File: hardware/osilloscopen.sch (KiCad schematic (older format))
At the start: 59 parts, among them J1 SWD, J10 Conn_01x01_Male, J11 Conn_01x02_Male, J12 Conn_01x03_Male, J13 Conn_01x02_Male, J14 Conn_01x02_Male, J15 Conn_01x01_Male, J16 Conn_01x03_Male, J17 OLED, J18 GND, J19 VBAT, J2 OLED, J3 tip, J4 power, J5 Conn_01x03_Male, J6 Conn_01x01_Male, J7 Conn_01x04_Male, J8 Conn_01x01_Male, J9 Conn_01x03_Male, SW1 SW_Push, SW2 SW_Push, SW3 SW_Push, SW4 SW_Push, SW5 POWER, SW6 RESET, U1 AD623AN, U2 ICL7660, U3 STM32F103C8Tx, U4 AP1117-33, U5 XXX, Y1 Crystal

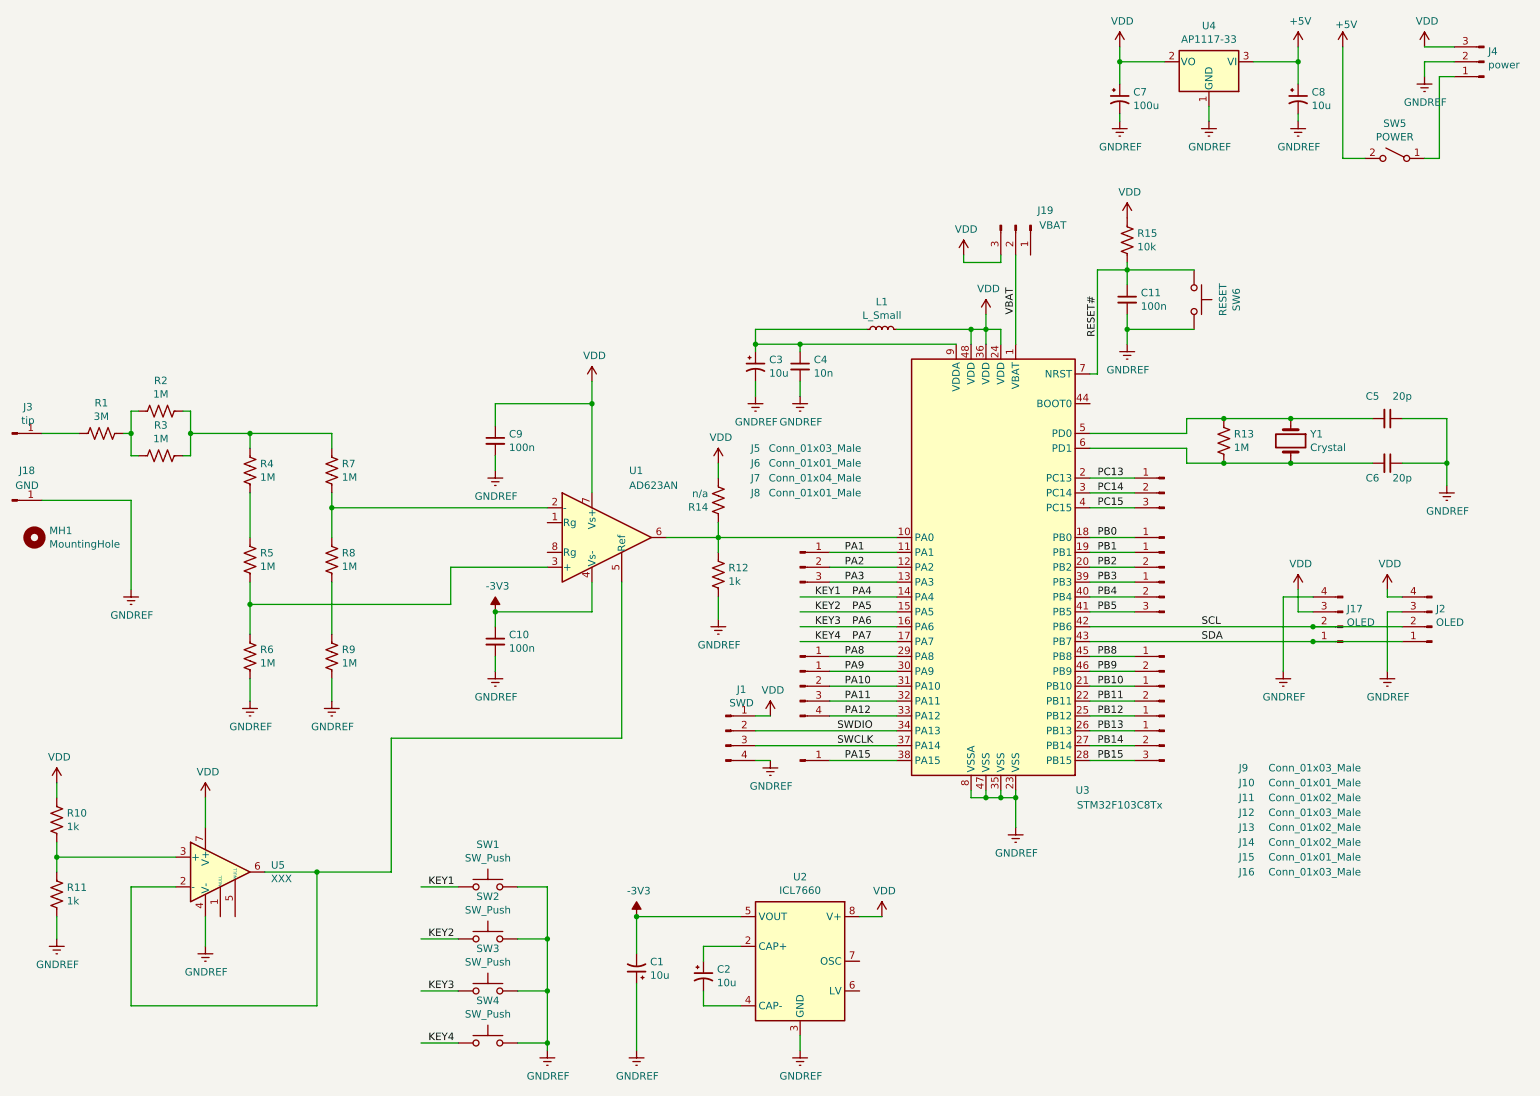
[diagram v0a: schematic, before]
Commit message: Add files via upload
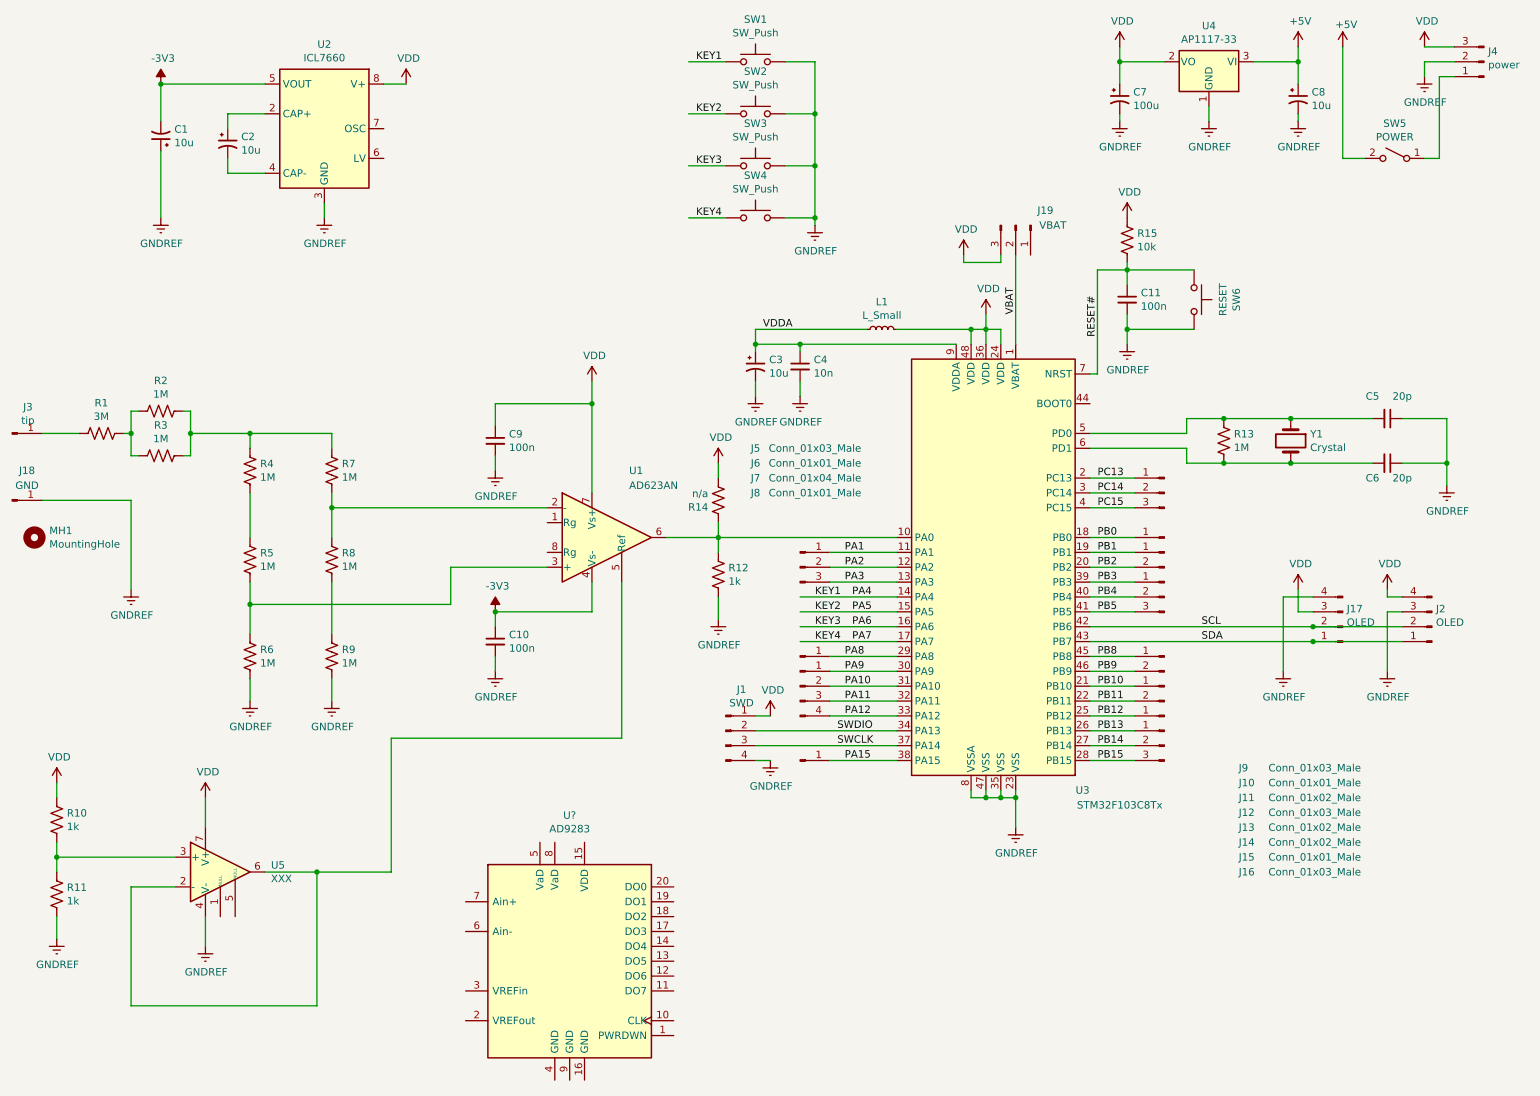
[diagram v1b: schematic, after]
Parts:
- added U?: AD9283, symbol Analog_ADC:AD9283
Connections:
- net labels added: VDDA
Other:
- moved on the sheet: C1, C2, SW1, SW2, SW3, SW4, U2
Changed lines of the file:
@@
 EESchema Schematic File Version 4
-LIBS:osilloscopen-cache
-EELAYER 26 0
+EELAYER 30 0
 EELAYER END
 $Descr A4 11693 8268
@@
 L Regulator_SwitchedCapacitor:ICL7660 U2
 U 1 1 5BCEDF67
-P 6300 6950
-F 0 "U2" H 6300 7517 50  0000 C CNN
-F 1 "ICL7660" H 6300 7426 50  0000 C CNN
-F 2 "Package_DIP:DIP-8_W7.62mm_LongPads" H 6400 6850 50  0001 C CNN
-F 3 "http://datasheets.maximintegrated.com/en/ds/ICL7660-MAX1044.pdf" H 6400 6850 50  0001 C CNN
-	1    6300 6950
+P 3100 1350
+F 0 "U2" H 3100 1917 50  0000 C CNN
+F 1 "ICL7660" H 3100 1826 50  0000 C CNN
+F 2 "Package_DIP:DIP-8_W7.62mm_LongPads" H 3200 1250 50  0001 C CNN
+F 3 "http://datasheets.maximintegrated.com/en/ds/ICL7660-MAX1044.pdf" H 3200 1250 50  0001 C CNN
+	1    3100 1350
 	-1   0    0    -1
 $EndComp
 Wire Wire Line
-	6700 6650 6850 6650
+	3500 1050 3650 1050
 $Comp
 L power:GNDREF #PWR0103
@@
 L power:GNDREF #PWR0105
 U 1 1 5BCEEDE7
-P 6300 7550
-F 0 "#PWR0105" H 6300 7300 50  0001 C CNN
-F 1 "GNDREF" H 6305 7377 50  0000 C CNN
-F 2 "" H 6300 7550 50  0001 C CNN
-F 3 "" H 6300 7550 50  0001 C CNN
-	1    6300 7550
-	1    0    0    -1
-$EndComp
-Wire Wire Line
-	6300 7550 6300 7450
+P 3100 1950
+F 0 "#PWR0105" H 3100 1700 50  0001 C CNN
+F 1 "GNDREF" H 3105 1777 50  0000 C CNN
+F 2 "" H 3100 1950 50  0001 C CNN
+F 3 "" H 3100 1950 50  0001 C CNN
+	1    3100 1950
+	1    0    0    -1
+$EndComp
+Wire Wire Line
+	3100 1950 3100 1850
 $Comp
 L Device:CP1_Small C2
 U 1 1 5BCEF09D
-P 5650 7050
-F 0 "C2" H 5741 7096 50  0000 L CNN
-F 1 "10u" H 5741 7005 50  0000 L CNN
-F 2 "Capacitor_THT:CP_Radial_D6.3mm_P2.50mm" H 5650 7050 50  0001 C CNN
-F 3 "~" H 5650 7050 50  0001 C CNN
-	1    5650 7050
+P 2450 1450
+F 0 "C2" H 2541 1496 50  0000 L CNN
+F 1 "10u" H 2541 1405 50  0000 L CNN
+F 2 "Capacitor_THT:CP_Radial_D6.3mm_P2.50mm" H 2450 1450 50  0001 C CNN
+F 3 "~" H 2450 1450 50  0001 C CNN
+	1    2450 1450
 	1    0    0    -1
 $EndComp
@@
 L Device:CP1_Small C1
 U 1 1 5BCEF0E8
-P 5200 7000
-F 0 "C1" H 5109 6954 50  0000 R CNN
-F 1 "10u" H 5109 7045 50  0000 R CNN
-F 2 "Capacitor_THT:CP_Radial_D6.3mm_P2.50mm" H 5200 7000 50  0001 C CNN
-F 3 "~" H 5200 7000 50  0001 C CNN
-	1    5200 7000
+P 2000 1400
+F 0 "C1" H 1909 1354 50  0000 R CNN
+F 1 "10u" H 1909 1445 50  0000 R CNN
+F 2 "Capacitor_THT:CP_Radial_D6.3mm_P2.50mm" H 2000 1400 50  0001 C CNN
+F 3 "~" H 2000 1400 50  0001 C CNN
+	1    2000 1400
 	-1   0    0    1
 $EndComp
 Wire Wire Line
-	5900 6850 5650 6850
-Wire Wire Line
-	5650 6850 5650 6950
-Wire Wire Line
-	5900 7250 5650 7250
-Wire Wire Line
-	5650 7250 5650 7150
+	2700 1250 2450 1250
+Wire Wire Line
+	2450 1250 2450 1350
+Wire Wire Line
+	2700 1650 2450 1650
+Wire Wire Line
+	2450 1650 2450 1550
 $Comp
 L power:GNDREF #PWR0106
 U 1 1 5BCEFBEB
-P 5200 7550
-F 0 "#PWR0106" H 5200 7300 50  0001 C CNN
-F 1 "GNDREF" H 5205 7377 50  0000 C CNN
-F 2 "" H 5200 7550 50  0001 C CNN
-F 3 "" H 5200 7550 50  0001 C CNN
-	1    5200 7550
+P 2000 1950
+F 0 "#PWR0106" H 2000 1700 50  0001 C CNN
+F 1 "GNDREF" H 2005 1777 50  0000 C CNN
+F 2 "" H 2000 1950 50  0001 C CNN
+F 3 "" H 2000 1950 50  0001 C CNN
+	1    2000 1950
 	1    0    0    -1
 $EndComp
@@
 L power:VDD #PWR0109
 U 1 1 5BCF1ECC
-P 6850 6650
-F 0 "#PWR0109" H 6850 6500 50  0001 C CNN
-F 1 "VDD" H 6867 6823 50  0000 C CNN
-F 2 "" H 6850 6650 50  0001 C CNN
-F 3 "" H 6850 6650 50  0001 C CNN
-	1    6850 6650
+P 3650 1050
+F 0 "#PWR0109" H 3650 900 50  0001 C CNN
+F 1 "VDD" H 3667 1223 50  0000 C CNN
+F 2 "" H 3650 1050 50  0001 C CNN
+F 3 "" H 3650 1050 50  0001 C CNN
+	1    3650 1050
 	1    0    0    -1
 $EndComp
@@
 L Switch:SW_Push SW1
 U 1 1 5BD06E7F
-P 4200 6450
-F 0 "SW1" H 4200 6735 50  0000 C CNN
-F 1 "SW_Push" H 4200 6644 50  0000 C CNN
-F 2 "Button_Switch_THT:SW_PUSH_6mm_H5mm" H 4200 6650 50  0001 C CNN
-F 3 "" H 4200 6650 50  0001 C CNN
-	1    4200 6450
+P 6000 900
+F 0 "SW1" H 6000 1185 50  0000 C CNN
+F 1 "SW_Push" H 6000 1094 50  0000 C CNN
+F 2 "Button_Switch_THT:SW_PUSH_6mm_H5mm" H 6000 1100 50  0001 C CNN
+F 3 "" H 6000 1100 50  0001 C CNN
+	1    6000 900
 	1    0    0    -1
 $EndComp
@@
 L Switch:SW_Push SW2
 U 1 1 5BD06EF3
-P 4200 6800
-F 0 "SW2" H 4200 7085 50  0000 C CNN
-F 1 "SW_Push" H 4200 6994 50  0000 C CNN
-F 2 "Button_Switch_THT:SW_PUSH_6mm_H5mm" H 4200 7000 50  0001 C CNN
-F 3 "" H 4200 7000 50  0001 C CNN
-	1    4200 6800
+P 6000 1250
+F 0 "SW2" H 6000 1535 50  0000 C CNN
+F 1 "SW_Push" H 6000 1444 50  0000 C CNN
+F 2 "Button_Switch_THT:SW_PUSH_6mm_H5mm" H 6000 1450 50  0001 C CNN
+F 3 "" H 6000 1450 50  0001 C CNN
+	1    6000 1250
 	1    0    0    -1
 $EndComp
@@
 L Switch:SW_Push SW3
 U 1 1 5BD06F40
-P 4200 7150
-F 0 "SW3" H 4200 7435 50  0000 C CNN
-F 1 "SW_Push" H 4200 7344 50  0000 C CNN
-F 2 "Button_Switch_THT:SW_PUSH_6mm_H5mm" H 4200 7350 50  0001 C CNN
-F 3 "" H 4200 7350 50  0001 C CNN
-	1    4200 7150
+P 6000 1600
+F 0 "SW3" H 6000 1885 50  0000 C CNN
+F 1 "SW_Push" H 6000 1794 50  0000 C CNN
+F 2 "Button_Switch_THT:SW_PUSH_6mm_H5mm" H 6000 1800 50  0001 C CNN
+F 3 "" H 6000 1800 50  0001 C CNN
+	1    6000 1600
 	1    0    0    -1
 $EndComp
@@
 L Switch:SW_Push SW4
 U 1 1 5BD06F8D
-P 4200 7500
-F 0 "SW4" H 4200 7785 50  0000 C CNN
-F 1 "SW_Push" H 4200 7694 50  0000 C CNN
-F 2 "Button_Switch_THT:SW_PUSH_6mm_H5mm" H 4200 7700 50  0001 C CNN
-F 3 "" H 4200 7700 50  0001 C CNN
-	1    4200 7500
-	1    0    0    -1
-$EndComp
-Wire Wire Line
-	4400 6450 4600 6450
-Wire Wire Line
-	4600 6450 4600 6800
-Wire Wire Line
-	4400 7500 4600 7500
-Connection ~ 4600 7500
-Wire Wire Line
-	4600 7500 4600 7550
-Wire Wire Line
-	4400 7150 4600 7150
-Connection ~ 4600 7150
-Wire Wire Line
-	4600 7150 4600 7500
-Wire Wire Line
-	4400 6800 4600 6800
-Connection ~ 4600 6800
-Wire Wire Line
-	4600 6800 4600 7150
+P 6000 1950
+F 0 "SW4" H 6000 2235 50  0000 C CNN
+F 1 "SW_Push" H 6000 2144 50  0000 C CNN
+F 2 "Button_Switch_THT:SW_PUSH_6mm_H5mm" H 6000 2150 50  0001 C CNN
+F 3 "" H 6000 2150 50  0001 C CNN
+	1    6000 1950
+	1    0    0    -1
+$EndComp
+Wire Wire Line
+	6200 900  6400 900
+Wire Wire Line
+	6400 900  6400 1250
+Wire Wire Line
+	6200 1950 6400 1950
+Connection ~ 6400 1950
+Wire Wire Line
+	6400 1950 6400 2000
+Wire Wire Line
+	6200 1600 6400 1600
+Connection ~ 6400 1600
+Wire Wire Line
+	6400 1600 6400 1950
+Wire Wire Line
+	6200 1250 6400 1250
+Connection ~ 6400 1250
+Wire Wire Line
+	6400 1250 6400 1600
 $Comp
 L power:GNDREF #PWR08
 U 1 1 5BD113E8
-P 4600 7550
-F 0 "#PWR08" H 4600 7300 50  0001 C CNN
-F 1 "GNDREF" H 4605 7377 50  0000 C CNN
-F 2 "" H 4600 7550 50  0001 C CNN
-F 3 "" H 4600 7550 50  0001 C CNN
-	1    4600 7550
-	1    0    0    -1
-$EndComp
-Wire Wire Line
-	4000 6450 3750 6450
-Wire Wire Line
-	4000 6800 3750 6800
-Wire Wire Line
-	4000 7150 3750 7150
-Wire Wire Line
-	4000 7500 3750 7500
-Text Label 3800 6450 0    50   ~ 0
+P 6400 2000
+F 0 "#PWR08" H 6400 1750 50  0001 C CNN
+F 1 "GNDREF" H 6405 1827 50  0000 C CNN
+F 2 "" H 6400 2000 50  0001 C CNN
+F 3 "" H 6400 2000 50  0001 C CNN
+	1    6400 2000
+	1    0    0    -1
+$EndComp
+Wire Wire Line
+	5800 900  5550 900
+Wire Wire Line
+	5800 1250 5550 1250
+Wire Wire Line
+	5800 1600 5550 1600
+Wire Wire Line
+	5800 1950 5550 1950
+Text Label 5600 900  0    50   ~ 0
 KEY1
-Text Label 3800 6800 0    50   ~ 0
+Text Label 5600 1250 0    50   ~ 0
 KEY2
-Text Label 3800 7150 0    50   ~ 0
+Text Label 5600 1600 0    50   ~ 0
 KEY3
-Text Label 3800 7500 0    50   ~ 0
+Text Label 5600 1950 0    50   ~ 0
 KEY4
 $Comp
@@
 L power:-3V3 #PWR0112
 U 1 1 5BD44E78
-P 5200 6650
-F 0 "#PWR0112" H 5200 6750 50  0001 C CNN
-F 1 "-3V3" H 5215 6823 50  0000 C CNN
-F 2 "" H 5200 6650 50  0001 C CNN
-F 3 "" H 5200 6650 50  0001 C CNN
-	1    5200 6650
+P 2000 1050
+F 0 "#PWR0112" H 2000 1150 50  0001 C CNN
+F 1 "-3V3" H 2015 1223 50  0000 C CNN
+F 2 "" H 2000 1050 50  0001 C CNN
+F 3 "" H 2000 1050 50  0001 C CNN
+	1    2000 1050
 	1    0    0    -1
 $EndComp
@@
 	8500 2300 8950 2300
 Wire Wire Line
-	5200 7550 5200 7100
-Wire Wire Line
-	5200 6900 5200 6650
+	2000 1950 2000 1500
+Wire Wire Line
+	2000 1300 2000 1050
 $Comp
 L power:-3V3 #PWR0115
@@
 $EndComp
 Connection ~ 4250 4600
-Connection ~ 5200 6650
-Wire Wire Line
-	5200 6650 5900 6650
+Connection ~ 2000 1050
+Wire Wire Line
+	2000 1050 2700 1050
 $Comp
 L Connector:Conn_01x03_Male J19
@@
 	3550 5450 5100 5450
 Connection ~ 3050 6350
+Text Label 6050 2700 0    50   ~ 0
+VDDA
+$Comp
+L Analog_ADC:AD9283 U?
+U 1 1 5FEBA64B
+P 4750 6950
+F 0 "U?" H 4750 7931 50  0000 C CNN
+F 1 "AD9283" H 4750 7840 50  0000 C CNN
+F 2 "" H 4750 6950 50  0001 C CNN
+F 3 "https://www.analog.com/media/en/technical-documentation/data-sheets/AD9283.pdf" H 4750 6950 50  0001 C CNN
+	1    4750 6950
+	1    0    0    -1
+$EndComp
 $EndSCHEMATC
